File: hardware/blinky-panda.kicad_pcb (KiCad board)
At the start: 2 copper layers, 69.5 x 56.4 mm, 36 parts, among them J1 AVR-ISP-6, SW1 SW_SPDT, SW2 SW_Push, U1 ATtiny84A-PU

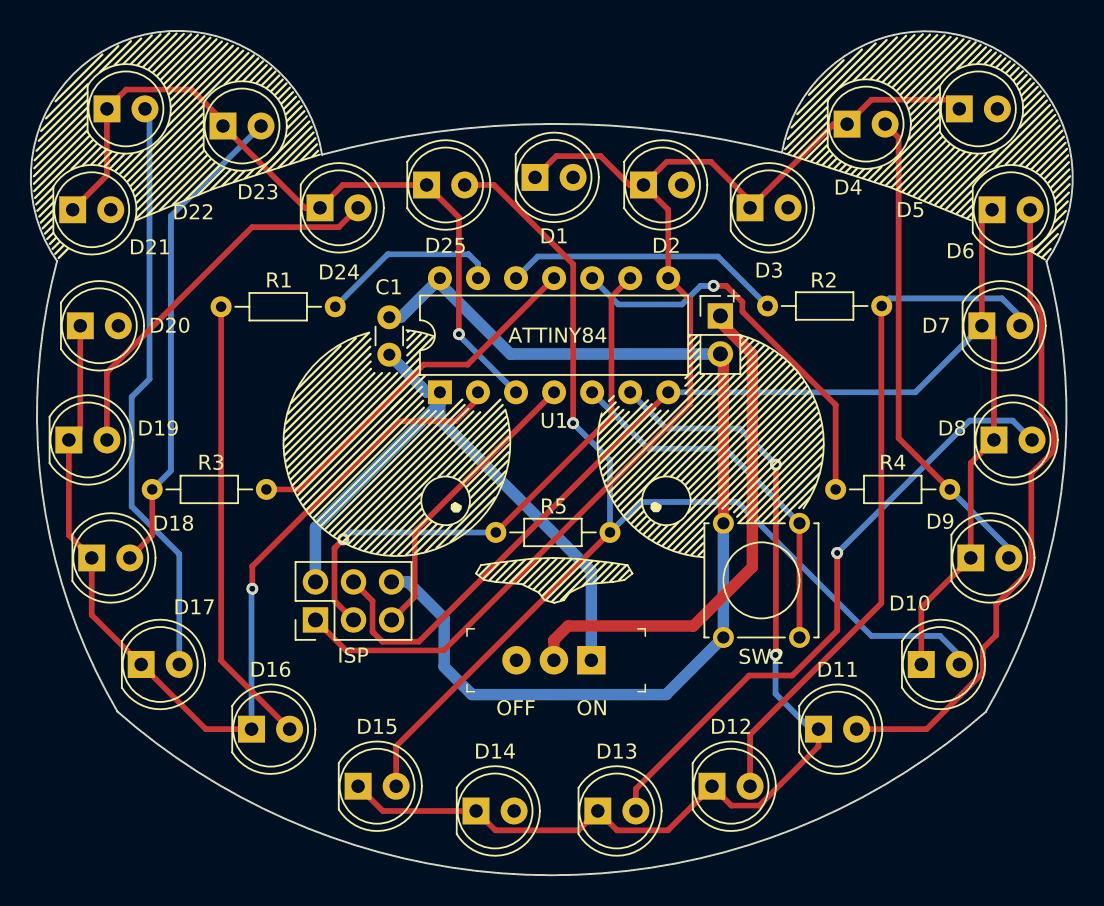
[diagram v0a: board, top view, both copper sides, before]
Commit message: complete circuit
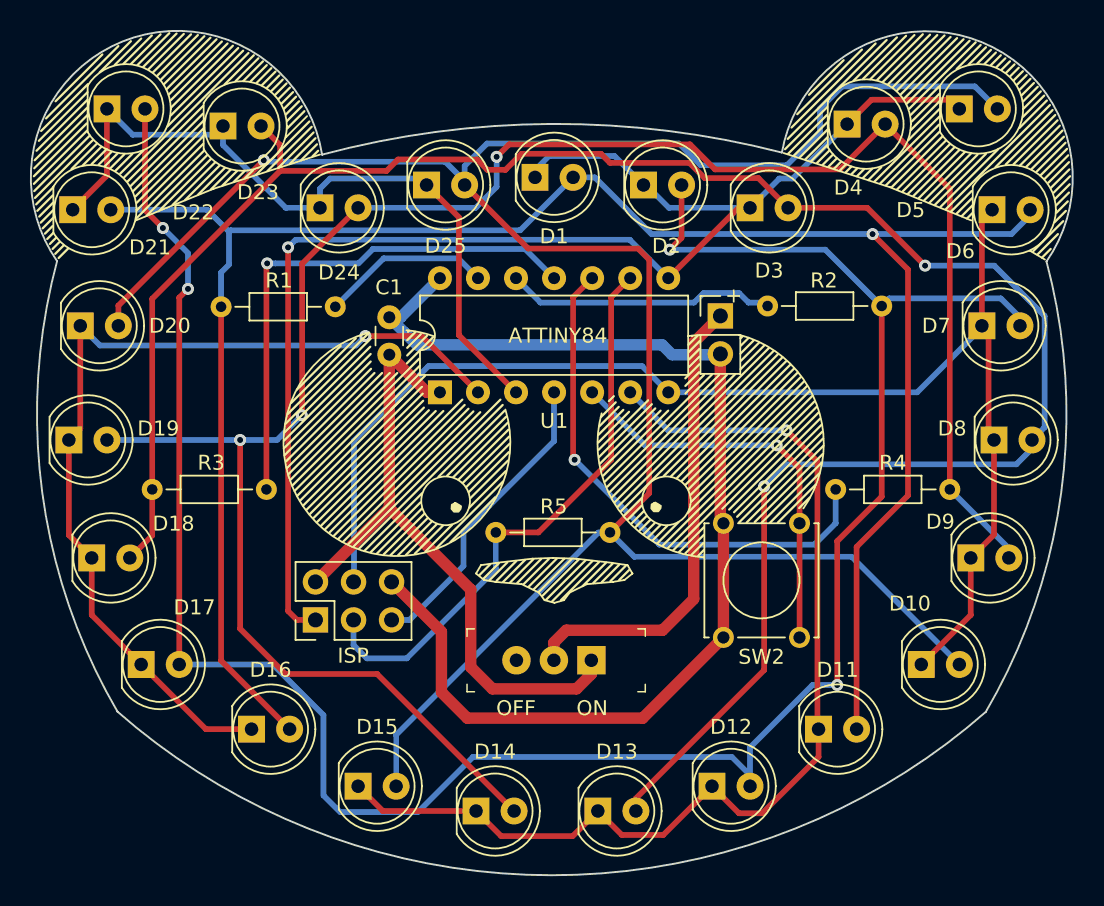
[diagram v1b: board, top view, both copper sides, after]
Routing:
- net Net-(D14-Pad2): track 58.2 -> 137.4 mm, vias 0 -> 3
- net Net-(D10-Pad2): track 80.2 -> 155.0 mm
- net Net-(D13-Pad2): track 74.1 -> 143.4 mm, vias 1 -> 2
- net Net-(D12-Pad2): track 85.3 -> 154.1 mm, vias 0 -> 4
- net Net-(D1-Pad2): track 73.6 -> 136.7 mm, vias 0 -> 1
- net /col4: track 83.7 -> 94.3 mm, vias 0 -> 1
- net /row2: track 25.0 -> 35.5 mm, vias 0 -> 1
- net /row3: track 26.8 -> 35.3 mm
- net GND: track 73.3 -> 77.1 mm
- net Net-(BT1-Pad1): track 34.8 -> 31.4 mm
- net /col2: track 68.4 -> 71.3 mm, vias 2 -> 1
- net /col3: track 86.5 -> 89.0 mm
- net /sw: track 25.1 -> 27.2 mm, vias 0 -> 1
- net /col1: track 65.1 -> 63.0 mm
- net VCC: track 42.6 -> 44.5 mm
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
